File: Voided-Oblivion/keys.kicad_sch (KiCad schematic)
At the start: 60 parts

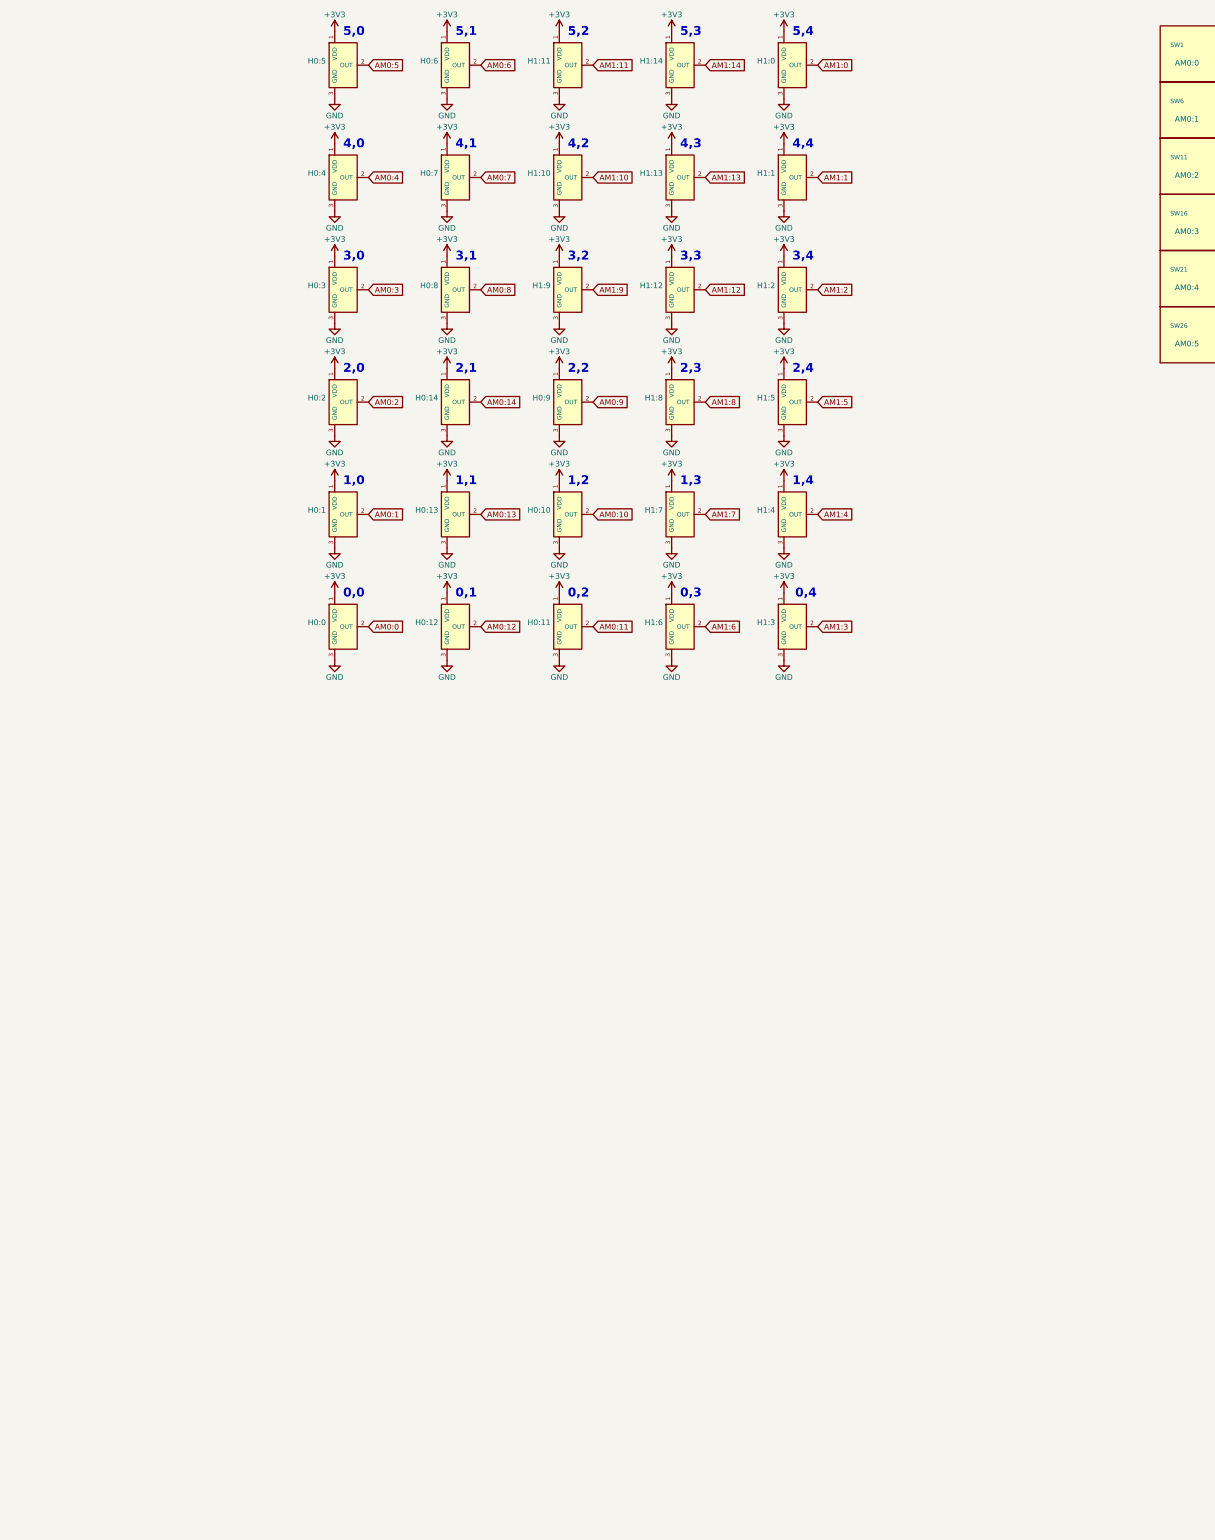
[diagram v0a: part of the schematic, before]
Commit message: update.com
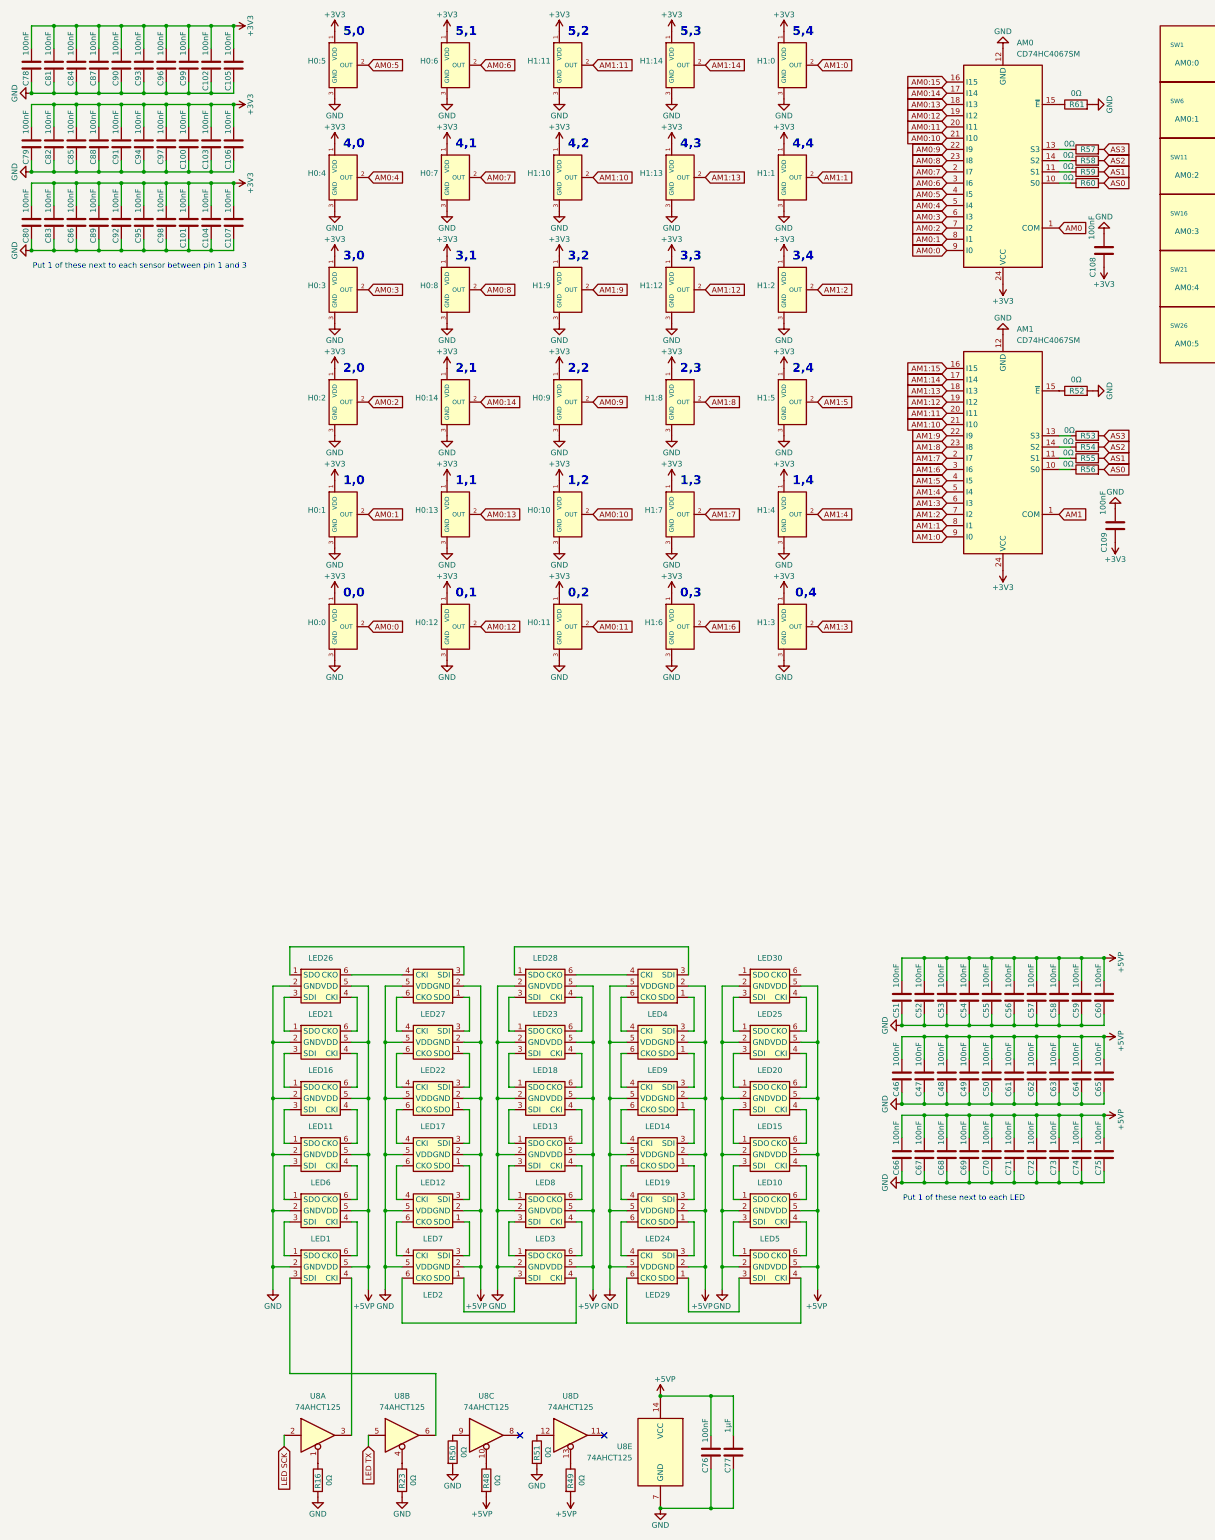
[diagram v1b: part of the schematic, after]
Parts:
- added AM0, AM1: CD74HC4067SM, Package_SO:SSOP-24_5.3x8.2mm_P0.65mm, symbol 74xx:CD74HC4067SM
- added C100, C101, C102, C103, C104, C105, C106, C107, C108, C109, C46, C47, C48, C49, C50, C51, C52, C53, C54, C55, C56, C57, C58, C59, C60, C61, C62, C63, C64, C65, C66, C67, C68, C69, C70, C71, C72, C73, C74, C75, C76, C78, C79, C80, C81, C82, C83, C84, C85, C86, C87, C88, C89, C90, C91, C92, C93, C94, C95, C96, C97, C98, C99: 100nF, Capacitor_SMD:C_0402_1005Metric, symbol Device:C
- added C77: 1µF, Capacitor_SMD:C_0402_1005Metric, symbol Device:C
- added LED1, LED10, LED11, LED12, LED13, LED14, LED15, LED16, LED17, LED18, LED19, LED2, LED20, LED21, LED22, LED23, LED24, LED25, LED26, LED27, LED28, LED29, LED3, LED30, LED4, LED5, LED6, LED7, LED8, LED9: (no value), SK9822-EC20:SK9822-EC20, symbol sk9822-ec20:SK9822-EC20
- added R16, R23, R48, R49, R50, R51, R52, R53, R54, R55, R56, R57, R58, R59, R60, R61: 0Ω, Resistor_SMD:R_0402_1005Metric, symbol Device:R
- added U8: 74AHCT125, symbol 74xx:74AHCT125
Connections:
- net +3V3: now also AM0.24 (VCC), AM1.24 (VCC), C100.2, C101.2, C102.2, C103.2, C104.2, C105.2, C106.2, C107.2, C108.1, C109.1, C78.2, C79.2, C80.2, C81.2, C82.2, C83.2, C84.2, C85.2, C86.2, C87.2, C88.2, C89.2, C90.2, C91.2, C92.2, C93.2, C94.2, C95.2, C96.2, C97.2, C98.2, C99.2
- net AM0:0: now also AM0.9 (I0)
- net AM0:1: now also AM0.8 (I1)
- net AM0:10: now also AM0.21 (I10)
- net AM0:11: now also AM0.20 (I11)
- net AM0:12: now also AM0.19 (I12)
- net AM0:13: now also AM0.18 (I13)
- net AM0:14: now also AM0.17 (I14)
- net AM0:2: now also AM0.7 (I2)
- net AM0:3: now also AM0.6 (I3)
- net AM0:4: now also AM0.5 (I4)
- net AM0:5: now also AM0.4 (I5)
- net AM0:6: now also AM0.3 (I6)
- net AM0:7: now also AM0.2 (I7)
- net AM0:8: now also AM0.23 (I8)
- net AM0:9: now also AM0.22 (I9)
- net AM1:0: now also AM1.9 (I0)
- net AM1:1: now also AM1.8 (I1)
- net AM1:10: now also AM1.21 (I10)
- net AM1:11: now also AM1.20 (I11)
- net AM1:12: now also AM1.19 (I12)
- net AM1:13: now also AM1.18 (I13)
- net AM1:14: now also AM1.17 (I14)
- net AM1:2: now also AM1.7 (I2)
- net AM1:3: now also AM1.6 (I3)
- net AM1:4: now also AM1.5 (I4)
- net AM1:5: now also AM1.4 (I5)
- net AM1:6: now also AM1.3 (I6)
- net AM1:7: now also AM1.2 (I7)
- net AM1:8: now also AM1.23 (I8)
- net AM1:9: now also AM1.22 (I9)
- net GND: now also AM0.12 (GND), AM1.12 (GND), C100.1, C101.1, C102.1, C103.1, C104.1, C105.1, C106.1, C107.1, C108.2, C109.2, C46.1, C47.1, C48.1, C49.1, C50.1, C51.1, C52.1, C53.1, C54.1, C55.1, C56.1, C57.1, C58.1, C59.1, C60.1, C61.1, C62.1, C63.1, C64.1, C65.1, C66.1, C67.1, C68.1, C69.1, C70.1, C71.1, C72.1, C73.1, C74.1, C75.1, C76.1, C77.1, C78.1, C79.1, C80.1, C81.1, C82.1, C83.1, C84.1, C85.1, C86.1, C87.1, C88.1, C89.1, C90.1, C91.1, C92.1, C93.1, C94.1, C95.1, C96.1, C97.1, C98.1, C99.1, LED1.2 (GND), LED10.2 (GND), LED11.2 (GND), LED12.5 (VDD), LED13.2 (GND), LED14.5 (VDD), LED15.2 (GND), LED16.2 (GND), LED17.5 (VDD), LED18.2 (GND), LED19.5 (VDD), LED2.5 (VDD), LED20.2 (GND), LED21.2 (GND), LED22.5 (VDD), LED23.2 (GND), LED24.5 (VDD), LED25.2 (GND), LED26.2 (GND), LED27.5 (VDD), LED28.2 (GND), LED29.5 (VDD), LED3.2 (GND), LED30.2 (GND), LED4.5 (VDD), LED5.2 (GND), LED6.2 (GND), LED7.5 (VDD), LED8.2 (GND), LED9.5 (VDD), R16.2, R23.2, R50.2, R51.2, R52.2, R61.2, U8.7 (GND)
- new net: LED13.3 (SDI), LED8.1 (SDO)
- new net: LED3.1 (SDO), LED8.3 (SDI)
- new net: LED3.6 (CKO), LED8.4 (CKI)
- new net: LED13.4 (CKI), LED8.6 (CKO)
- new net: LED13.1 (SDO), LED18.3 (SDI)
- new net: LED13.6 (CKO), LED18.4 (CKI)
- new net: LED14.1 (SDO), LED19.3 (SDI)
- new net: LED14.3 (SDI), LED9.1 (SDO)
- new net: LED14.4 (CKI), LED9.6 (CKO)
- new net: LED14.6 (CKO), LED19.4 (CKI)
- new net: R23.1, U8.4
- new net: AM0.10 (S0), R60.1
- new net: LED25.1 (SDO), LED30.3 (SDI)
- new net: LED25.6 (CKO), LED30.4 (CKI)
- new net: R51.1, U8.12
- new net: LED12.1 (SDO), LED7.3 (SDI)
- new net: LED12.3 (SDI), LED17.1 (SDO)
- new net: LED12.4 (CKI), LED17.6 (CKO)
- new net: LED12.6 (CKO), LED7.4 (CKI)
- new net: LED2.1 (SDO), LED3.3 (SDI)
- new net: LED2.3 (SDI), LED7.1 (SDO)
- new net: LED2.4 (CKI), LED7.6 (CKO)
- new net: LED2.6 (CKO), LED3.4 (CKI)
- new net: LED21.1 (SDO), LED26.3 (SDI)
- new net: LED16.1 (SDO), LED21.3 (SDI)
- new net: LED16.6 (CKO), LED21.4 (CKI)
- new net: LED21.6 (CKO), LED26.4 (CKI)
- new net: LED28.1 (SDO), LED4.3 (SDI)
- new net: LED23.1 (SDO), LED28.3 (SDI)
- new net: LED23.6 (CKO), LED28.4 (CKI)
- new net: LED28.6 (CKO), LED4.4 (CKI)
- new net: LED19.1 (SDO), LED24.3 (SDI)
- new net: LED19.6 (CKO), LED24.4 (CKI)
- new net: AM0.11 (S1), R59.1
- new net: AM0.13 (S3), R57.1
- new net: AM0.14 (S2), R58.1
- new net: AM0.15 (~{E}), R61.1
- new net: LED10.3 (SDI), LED5.1 (SDO)
- new net: LED29.1 (SDO), LED5.3 (SDI)
- new net: LED29.6 (CKO), LED5.4 (CKI)
- new net: LED10.4 (CKI), LED5.6 (CKO)
- new net: LED11.1 (SDO), LED16.3 (SDI)
- new net: LED11.3 (SDI), LED6.1 (SDO)
- new net: LED11.4 (CKI), LED6.6 (CKO)
- new net: LED11.6 (CKO), LED16.4 (CKI)
- new net: LED1.1 (SDO), LED6.3 (SDI)
- new net: LED1.3 (SDI), U8.6
- new net: LED1.4 (CKI), U8.3
- new net: LED1.6 (CKO), LED6.4 (CKI)
- new net: LED10.1 (SDO), LED15.3 (SDI)
- new net: LED10.6 (CKO), LED15.4 (CKI)
- new net: AM1.10 (S0), R56.1
- new net: AM1.11 (S1), R55.1
- new net: AM1.13 (S3), R53.1
- new net: AM1.14 (S2), R54.1
- new net: AM1.15 (~{E}), R52.1
- new net: LED20.1 (SDO), LED25.3 (SDI)
- new net: LED20.6 (CKO), LED25.4 (CKI)
- new net: LED15.1 (SDO), LED20.3 (SDI)
- new net: LED15.6 (CKO), LED20.4 (CKI)
- new net: LED24.1 (SDO), LED29.3 (SDI)
- new net: LED24.6 (CKO), LED29.4 (CKI)
- new net: LED17.3 (SDI), LED22.1 (SDO)
- new net: LED22.3 (SDI), LED27.1 (SDO)
- new net: LED22.4 (CKI), LED27.6 (CKO)
- new net: LED17.4 (CKI), LED22.6 (CKO)
- new net: R48.1, U8.10
- new net: R49.1, U8.13
- new net: LED26.1 (SDO), LED27.3 (SDI)
- new net: LED26.6 (CKO), LED27.4 (CKI)
- new net: R50.1, U8.9
- new net: LED18.1 (SDO), LED23.3 (SDI)
- new net: LED18.6 (CKO), LED23.4 (CKI)
- new net: R16.1, U8.1
- new net: LED4.1 (SDO), LED9.3 (SDI)
- new net: LED4.6 (CKO), LED9.4 (CKI)
- new net +5VP: C46.2, C47.2, C48.2, C49.2, C50.2, C51.2, C52.2, C53.2, C54.2, C55.2, C56.2, C57.2, C58.2, C59.2, C60.2, C61.2, C62.2, C63.2, C64.2, C65.2, C66.2, C67.2, C68.2, C69.2, C70.2, C71.2, C72.2, C73.2, C74.2, C75.2, C76.2, C77.2, LED1.5 (VDD), LED10.5 (VDD), LED11.5 (VDD), LED12.2 (GND), LED13.5 (VDD), LED14.2 (GND), LED15.5 (VDD), LED16.5 (VDD), LED17.2 (GND), LED18.5 (VDD), LED19.2 (GND), LED2.2 (GND), LED20.5 (VDD), LED21.5 (VDD), LED22.2 (GND), LED23.5 (VDD), LED24.2 (GND), LED25.5 (VDD), LED26.5 (VDD), LED27.2 (GND), LED28.5 (VDD), LED29.2 (GND), LED3.5 (VDD), LED30.5 (VDD), LED4.2 (GND), LED5.5 (VDD), LED6.5 (VDD), LED7.2 (GND), LED8.5 (VDD), LED9.2 (GND), R48.2, R49.2, U8.14 (VCC)
- new net AM0: AM0.1 (COM)
- new net AM0:15: AM0.16 (I15)
- new net AM1: AM1.1 (COM)
- new net AM1:15: AM1.16 (I15)
- new net AS0: R56.2, R60.2
- new net AS1: R55.2, R59.2
- new net AS2: R54.2, R58.2
- new net AS3: R53.2, R57.2
- new net LED SCK: U8.2
- new net LED TX: U8.5
- no-connect marks 0 -> 2
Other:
- note added: "Put 1 of these next to each LED"
- note added: "Put 1 of these next to each sensor between pin 1 and 3"
